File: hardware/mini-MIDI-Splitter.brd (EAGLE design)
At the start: 138.4 x 19 mm, 40 parts, among them IC1 6N138, IC2 4050D, IC3 REG1117, X1 DIN5PIN, X2 DIN5PIN, X3 DIN5PIN, X4 DIN5PIN, X5 DIN5PIN, X6 DIN5PIN

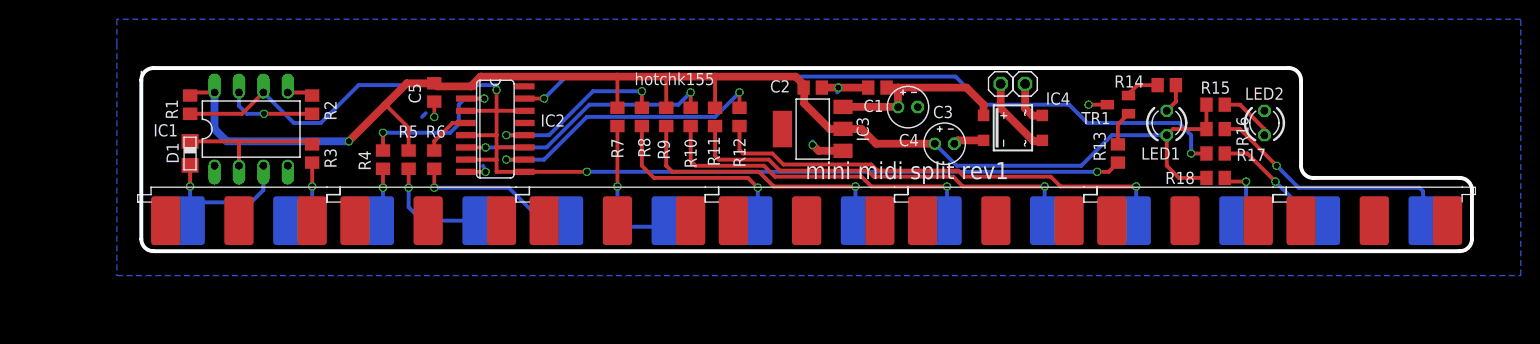
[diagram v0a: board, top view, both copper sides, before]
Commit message: updates
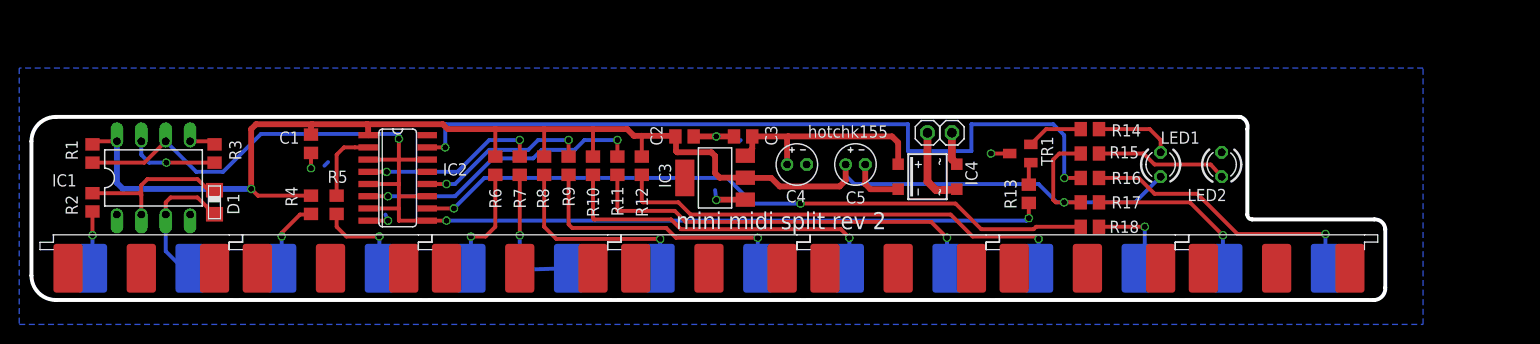
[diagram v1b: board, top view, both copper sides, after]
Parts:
- C3: device rcl:E2-4 -> rcl:C0805
- C5: device rcl:C0805 -> rcl:E2-4
- moved C1 59.2 mm to (29.1, 16.3), turned to 270 degrees
- moved C5 44.5 mm to (85.7, 14.1), turned to 0 degrees
- moved R2 25.0 mm to (6.35, 10.2), turned to 90 degrees
- moved C3 17.4 mm to (74.0, 17.0), turned to 180 degrees
- moved C4 15.5 mm to (79.6, 14.1)
- moved C2 14.3 mm to (67.9, 17.0)
- moved R15 14.0 mm to (110.1, 15.2)
- moved R16 14.0 mm to (110.1, 12.7), turned to 0 degrees
- moved R17 14.0 mm to (110.1, 10.2), turned to 180 degrees
- moved R18 14.0 mm to (110.1, 7.62), turned to 0 degrees
- moved R10 13.7 mm to (58.4, 14.0)
- moved R1 11.4 mm to (6.35, 15.2)
- moved R7 11.4 mm to (50.8, 14.0), turned to 270 degrees
- moved R9 11.4 mm to (55.9, 14.0), turned to 270 degrees
- moved IC1 11.4 mm to (12.7, 12.7)
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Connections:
- net GND: now also C3.2, C5.-, R3.1; no longer C3.-, C5.2, R2.1
- net N$1: now also R5.2; no longer R4.2
- net N$11: now also R7.1; no longer R6.1
- net N$12: now also R5.1; no longer R4.1
- net N$14: now also R4.1; no longer R5.1
- net N$15: now also R6.1; no longer R7.1
- net N$16: now also R8.1; no longer R9.1
- net N$18: now also R12.1; no longer R18.1
- net N$19: now also R17.1; no longer R16.1
- net N$2: now also R7.2; no longer R6.2
- net N$20: now also R2.1; no longer R3.1
- net N$21: now also R2.2; no longer R3.2
- net N$22: now also R3.2; no longer R2.2
- net N$3: now also R9.2; no longer R8.2
- net N$5: now also R18.2; no longer R12.2
- net N$6: now also R16.2; no longer R17.2
- net N$7: now also R16.1; no longer R17.1
- net N$8: now also R9.1; no longer R8.1
- net N$9: now also R18.1; no longer R12.1
- net VCC: now also C1.1, C5.+, R12.2, R17.2, R4.2, R6.2, R8.2; no longer C4.+, C5.1, R16.2, R18.2, R5.2, R7.2, R9.2
- net VIN: now also C3.1, C4.+; no longer C1.1, C3.+
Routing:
- net N$18: track 7.42 -> 48.7 mm
- net N$9: track 30.7 -> 71.6 mm
- net N$5: track 48.9 -> 9.49 mm
- net VCC: track 146.5 -> 162.4 mm, vias 1 -> 2
- net N$6: track 13.7 -> 29.5 mm
- net N$11: track 5.02 -> 18.9 mm, vias 0 -> 2
- net N$12: track 17.0 -> 7.85 mm, vias 2 -> 0
- net N$4: track 35.0 -> 43.1 mm
- net N$3: track 20.6 -> 28.6 mm
- net N$26: track 5.82 -> 13.8 mm
- net N$19: track 26.4 -> 19.2 mm
- net N$17: track 42.3 -> 35.2 mm
- net N$23: track 3.06 -> 8.16 mm
- net N$7: track 76.3 -> 80.9 mm
- net N$14: track 11.7 -> 7.55 mm
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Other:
- board size 138.4 x 19 mm -> 140.8 x 19.1 mm
- board text added: "mini midi split rev 2"
- board text removed: "mini midi split rev1"
